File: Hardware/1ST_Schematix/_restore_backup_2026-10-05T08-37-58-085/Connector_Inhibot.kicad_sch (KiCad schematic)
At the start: 19 parts, among them J511_OUT401 Conn_01x06, U401 LSM6DSL, U402 DRV8833PW

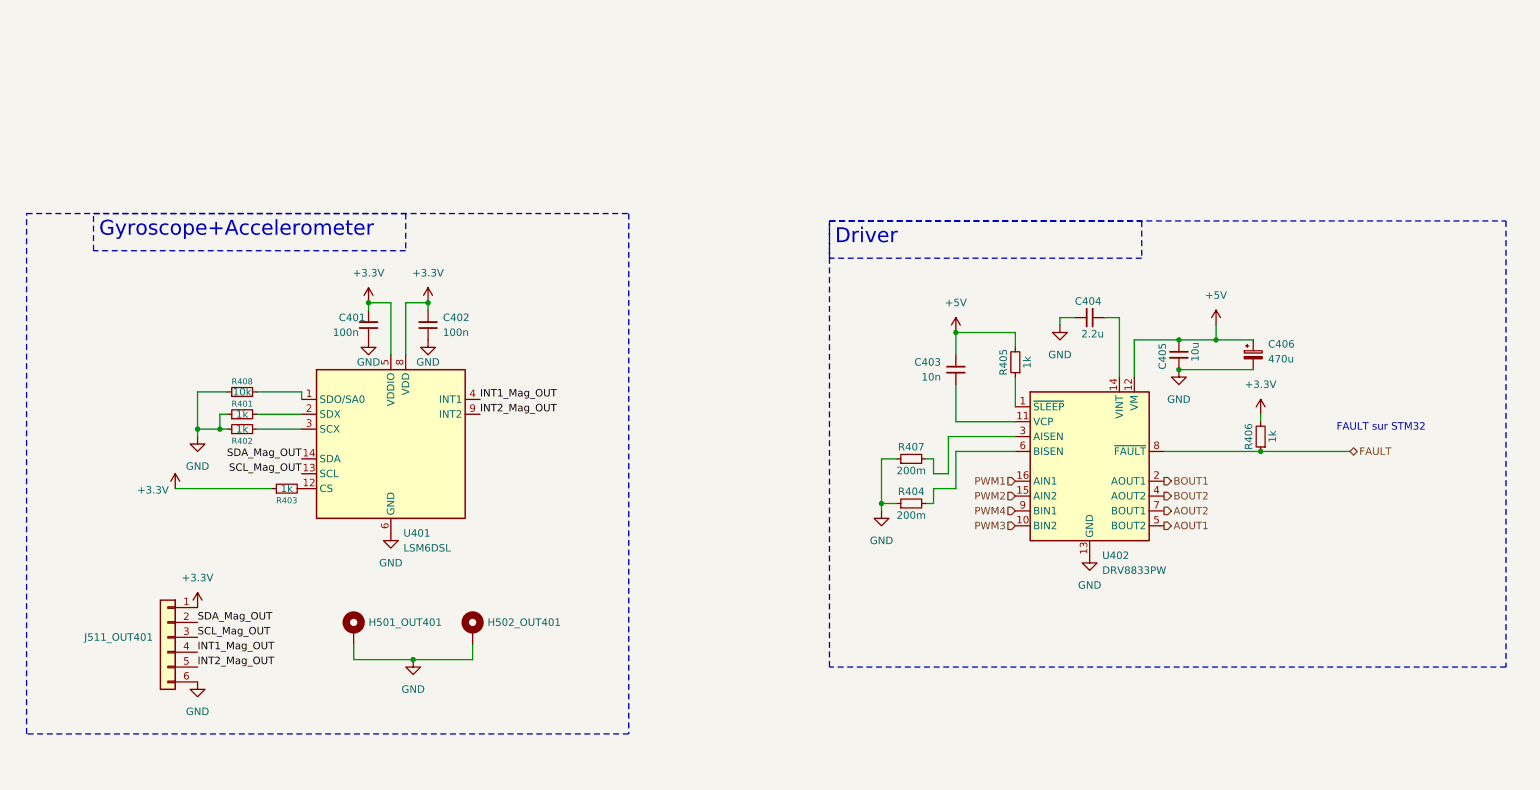
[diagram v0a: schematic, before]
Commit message: début du routing
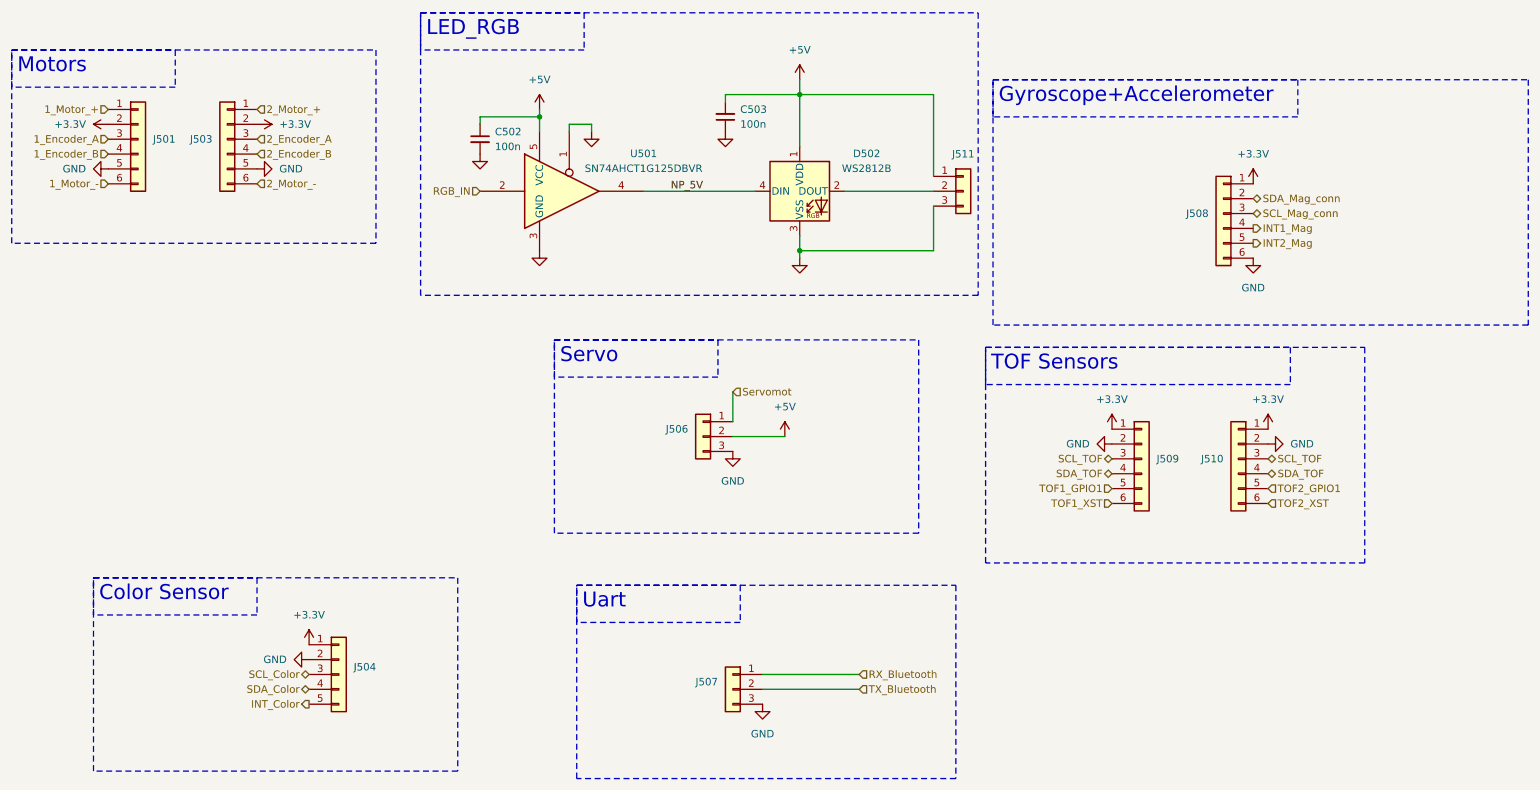
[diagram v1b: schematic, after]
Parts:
- removed C401, C402: 100n, Capacitor_SMD:C_0402_1005Metric, symbol Device:C_Small
- removed C403: 10n, Capacitor_SMD:C_0402_1005Metric, symbol Device:C_Small
- removed C404: 2.2u, Capacitor_SMD:C_0402_1005Metric, symbol Device:C_Small
- removed C405: 10u, Capacitor_SMD:C_0402_1005Metric, symbol Device:C_Small
- removed C406: 470u, Capacitor_SMD:CP_Elec_10x10.5, symbol Device:C_Polarized_Small
- removed H501_OUT401, H502_OUT401: MountingHole_Pad, MountingHole:MountingHole_3.2mm_M3_ISO14580_Pad, symbol Mechanical:MountingHole_Pad
- removed J511_OUT401: Conn_01x06, Connector_JST:JST_EH_B6B-EH-A_1x06_P2.50mm_Vertical, symbol Connector_Generic:Conn_01x06
- removed R401, R402, R403, R405, R406: 1k, Resistor_SMD:R_0402_1005Metric, symbol Device:R_Small
- removed R404, R407: 200m, Resistor_SMD:R_0805_2012Metric, symbol Device:R_Small
- removed R408: 10k, Resistor_SMD:R_0402_1005Metric, symbol Device:R_Small
- removed U401: LSM6DSL, Package_LGA:LGA-14_3x2.5mm_P0.5mm_LayoutBorder3x4y, symbol Sensor_Motion:LSM6DSL
- removed U402: DRV8833PW, Package_SO:TSSOP-16_4.4x5mm_P0.65mm, symbol Driver_Motor:DRV8833PW
- added C502, C503: 100n, Capacitor_SMD:C_0402_1005Metric, symbol Device:C_Small
- added D502: WS2812B, LED_SMD:LED_WS2812B-Mini_PLCC4_3.5x3.5mm, symbol LED:WS2812B
- added J501, J503, J508, J509, J510: Conn_01x06, Connector_JST:JST_EH_B6B-EH-A_1x06_P2.50mm_Vertical, symbol Connector_Generic:Conn_01x06
- added J504: Conn_01x05, Connector_JST:JST_EH_B5B-EH-A_1x05_P2.50mm_Vertical, symbol Connector_Generic:Conn_01x05
- added J506, J507, J511: Conn_01x03, Connector_JST:JST_EH_B3B-EH-A_1x03_P2.50mm_Vertical, symbol Connector_Generic:Conn_01x03
- added U501: SN74AHCT1G125DBVR, Package_TO_SOT_SMD:SOT-23-5, symbol 74xGxx:74AHCT1G125
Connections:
- net +3.3V: now also J501.2 (Pin_2), J503.2 (Pin_2), J504.1 (Pin_1), J508.1 (Pin_1), J509.1 (Pin_1), J510.1 (Pin_1)
- net +5V: now also C502.1, C503.2, D502.1 (VDD), J506.2 (Pin_2), J511.1 (Pin_1), U501.5 (VCC)
- net GND: now also C502.2, C503.1, D502.3 (VSS), J501.5 (Pin_5), J503.5 (Pin_5), J504.2 (Pin_2), J506.3 (Pin_3), J507.3 (Pin_3), J508.6 (Pin_6), J509.2 (Pin_2), J510.2 (Pin_2), J511.3 (Pin_3), U501.1, U501.3 (GND)
- new net: D502.2 (DOUT), J511.2 (Pin_2)
- new net 1_Encoder_A: J501.3 (Pin_3)
- new net 1_Encoder_B: J501.4 (Pin_4)
- new net 1_Motor_+: J501.1 (Pin_1)
- new net 1_Motor_-: J501.6 (Pin_6)
- new net 2_Encoder_A: J503.3 (Pin_3)
- new net 2_Encoder_B: J503.4 (Pin_4)
- new net 2_Motor_+: J503.1 (Pin_1)
- new net 2_Motor_-: J503.6 (Pin_6)
- new net INT1_Mag: J508.4 (Pin_4)
- new net INT2_Mag: J508.5 (Pin_5)
- new net INT_Color: J504.5 (Pin_5)
- new net NP_5V: D502.4 (DIN), U501.4
- new net RGB_IN: U501.2
- new net RX_Bluetooth: J507.1 (Pin_1)
- new net SCL_Color: J504.3 (Pin_3)
- new net SCL_Mag_conn: J508.3 (Pin_3)
- new net SCL_TOF: J509.3 (Pin_3), J510.3 (Pin_3)
- new net SDA_Color: J504.4 (Pin_4)
- new net SDA_Mag_conn: J508.2 (Pin_2)
- new net SDA_TOF: J509.4 (Pin_4), J510.4 (Pin_4)
- new net Servomot: J506.1 (Pin_1)
- new net TOF1_GPIO1: J509.5 (Pin_5)
- new net TOF1_XST: J509.6 (Pin_6)
- new net TOF2_GPIO1: J510.5 (Pin_5)
- new net TOF2_XST: J510.6 (Pin_6)
- new net TX_Bluetooth: J507.2 (Pin_2)
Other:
- note removed: "FAULT sur STM32"
